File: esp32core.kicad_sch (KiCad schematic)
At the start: 1 part

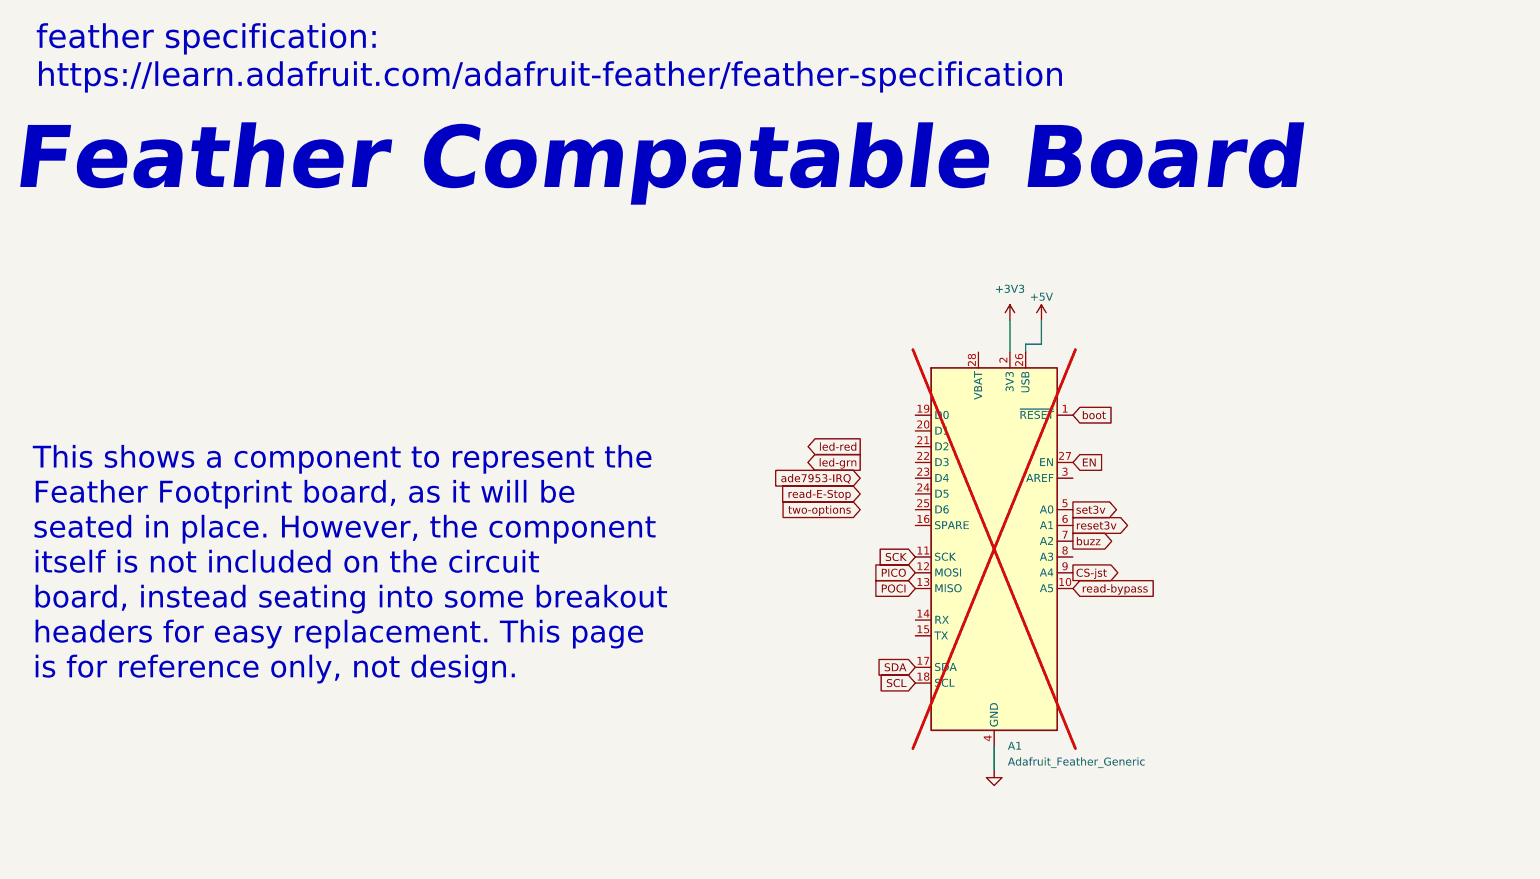
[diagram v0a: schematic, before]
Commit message: 1.4.1 schematic update
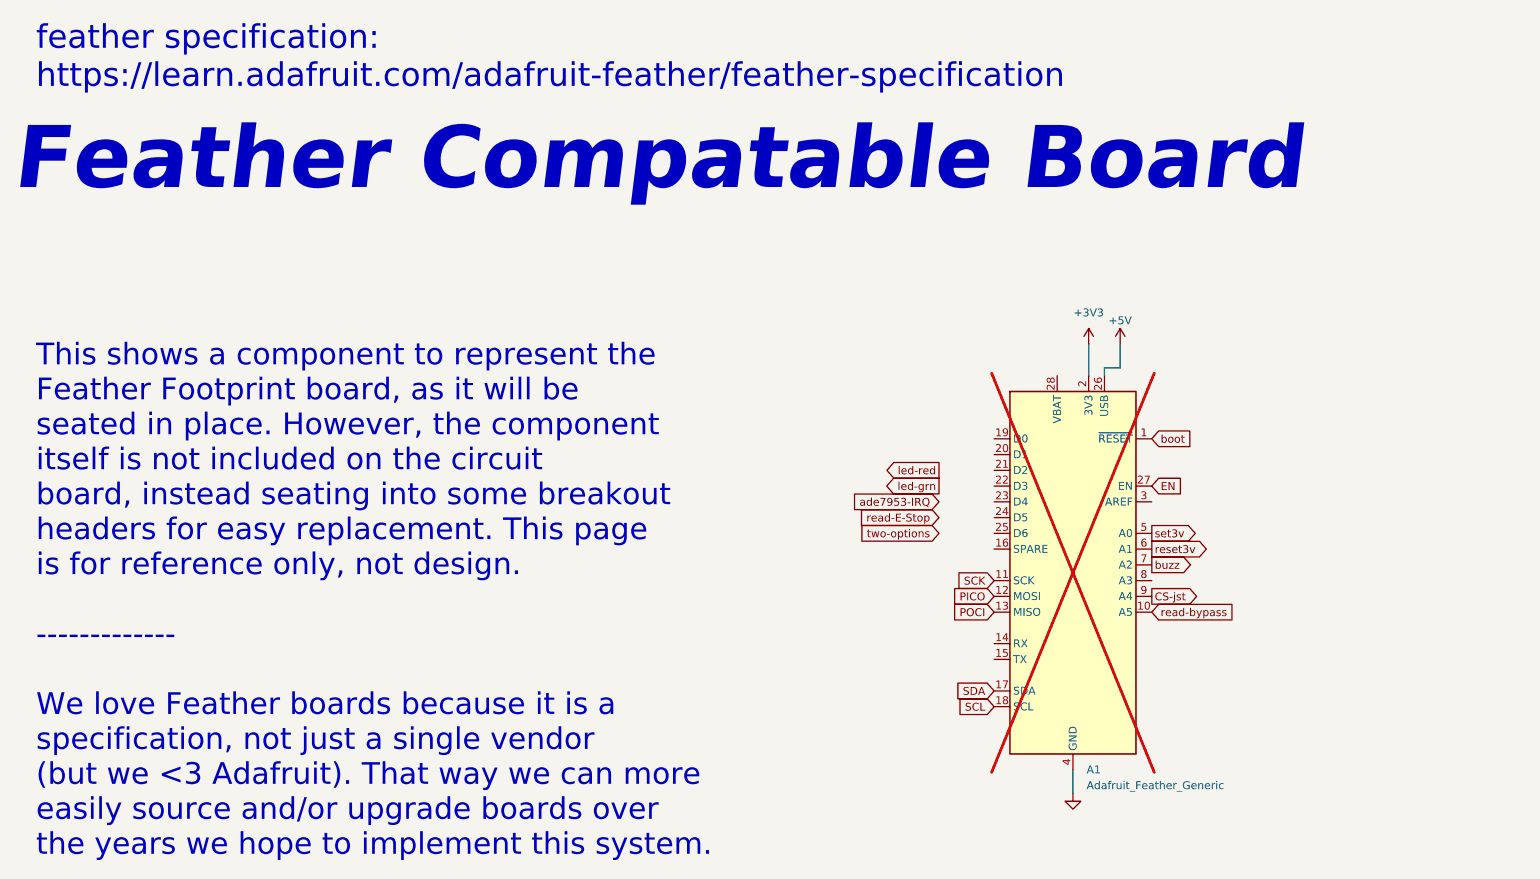
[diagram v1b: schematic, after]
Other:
- note added: "This shows a component to represent the Feather Footprint board, as it will be seated in place. However, the component itself is not included on the circuit board, instead seating into some breakout headers for easy replacement. This page is for reference only, not design. ------------- We love Feather boards because it is a specification, not just a single vendor (but we <3 Adafruit). That way w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"
- note removed: "This shows a component to represent the Feather Footprint board, as it will be seated in place. However, the component itself is not included on the circuit board, instead seating into some breakout headers for easy replacement. This page is for reference only, not design."
- moved on the sheet: A1
